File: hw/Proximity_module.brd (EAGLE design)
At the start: 25 x 45 mm, 44 parts, among them J1 GROVE-4P-2.0-3470130P1, J2 GROVE-4P-2.0-3470130P1, U5 LD3985XX, X1 53047-04, X2 53047-04, X3 53047-04, X4 53047-04, X5 53047-04, X6 53047-04, X7 53047-04, X8 53047-04

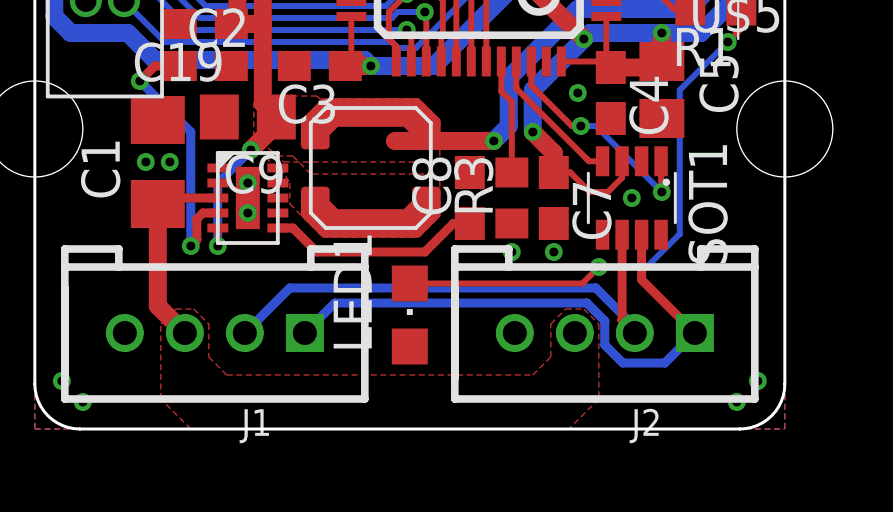
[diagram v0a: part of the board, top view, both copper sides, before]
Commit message: minor fixes for manufacturing
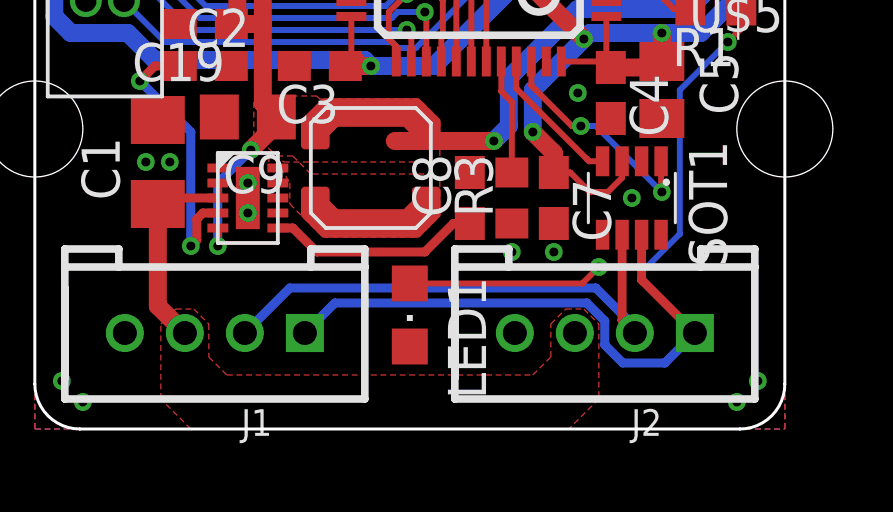
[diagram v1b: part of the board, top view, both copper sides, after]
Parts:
- turned LED1 to 180 degrees
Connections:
- net GND: now also LED1.C; no longer LED1.A
- net N$4: now also LED1.A; no longer LED1.C
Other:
- board text added: "Proximity module v1.1 (2014/12)"
- board text removed: "Proximity module rev 1.1"
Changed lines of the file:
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@@
 <layer number="50" name="dxf" color="7" fill="1" visible="no" active="no"/>
 <layer number="51" name="tDocu" color="7" fill="1" visible="no" active="yes"/>
-<layer number="52" name="bDocu" color="7" fill="1" visible="no" active="yes"/>
+<layer number="52" name="bDocu" color="7" fill="1" visible="yes" active="yes"/>
 <layer number="53" name="tGND_GNDA" color="7" fill="1" visible="no" active="no"/>
 <layer number="54" name="bGND_GNDA" color="7" fill="1" visible="no" active="no"/>
@@
 <wire x1="14.5" y1="26.9" x2="14.5" y2="28.5" width="0.1" layer="48"/>
 <text x="4" y="6" size="1.5" layer="200" rot="MR90">Proximity module
-rev 1.1</text>
+v1.1 (2014/12)</text>
 </plain>
 <attributes>
@@
 <element name="C3" library="rcl" package="C0603" value="100n" x="9.5" y="12.1" rot="R180"/>
 <element name="C7" library="rcl" package="C0603" value="100n" x="17.3" y="7.7" rot="R270"/>
-<element name="LED1" library="led" package="CHIPLED_0805" value="" x="12.5" y="3.8"/>
+<element name="LED1" library="led" package="CHIPLED_0805" value="" x="12.5" y="3.8" rot="R180"/>
 <element name="R1" library="rcl" package="R0603" value="330" x="22.7" y="14" rot="R180"/>
 <element name="U$4" library="samtec" package="FTSH-105-TH" value="FTSH-105TH" x="1.7" y="16.8" rot="R270"/>
@@
 <via x="7.1" y="8.2" extent="1-16" drill="0.3"/>
 <via x="7.1" y="7.2" extent="1-16" drill="0.3"/>
-<contactref element="LED1" pad="A"/>
 <contactref element="SOT1" pad="2"/>
 <contactref element="SOT1" pad="8"/>
@@
 <via x="22" y="25.5" extent="1-16" drill="0.3"/>
 <via x="22" y="24.5" extent="1-16" drill="0.3"/>
+<contactref element="LED1" pad="C"/>
 </signal>
 <signal name="VIN">
@@
 <signal name="N$4">
 <contactref element="R1" pad="1"/>
-<contactref element="LED1" pad="C"/>
 <via x="23.1" y="12.9" extent="1-16" drill="0.3"/>
 <wire x1="23.55" y1="14" x2="23.55" y2="13.35" width="0.2" layer="1"/>
 <wire x1="23.55" y1="13.35" x2="23.1" y2="12.9" width="0.2" layer="1"/>
-<wire x1="12.5" y1="4.85" x2="18.25" y2="4.85" width="0.2" layer="1"/>
 <wire x1="18.25" y1="4.85" x2="18.8" y2="5.4" width="0.2" layer="1"/>
 <via x="18.8" y="5.4" extent="1-16" drill="0.3"/>
@@
 <wire x1="21.5" y1="6.5" x2="21.5" y2="11.3" width="0.2" layer="16"/>
 <wire x1="21.5" y1="11.3" x2="23.1" y2="12.9" width="0.2" layer="16"/>
+<contactref element="LED1" pad="A"/>
+<wire x1="18.25" y1="4.85" x2="12.5" y2="4.85" width="0.2" layer="1"/>
 </signal>
 <signal name="N$2">
